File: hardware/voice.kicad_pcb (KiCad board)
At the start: 2 copper layers, 111.8 x 50.8 mm, 56 parts, among them K1 PWR, P1 DATA, P2 OUT, U1 4051, U2 MCP4922-E/P, U3 MCP4922-E/P, U4 TL074, U5 SSM2044, U6 SSM2044

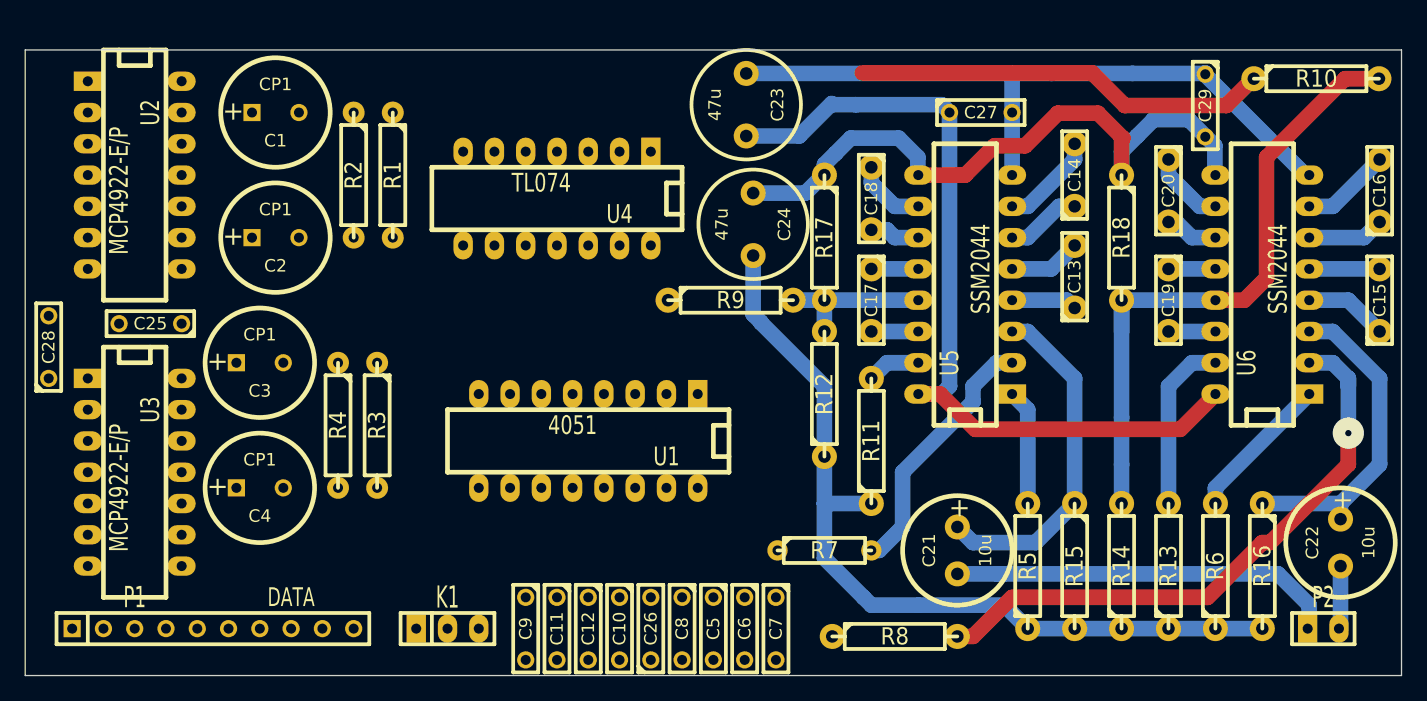
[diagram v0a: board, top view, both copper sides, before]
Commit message: hardware project cleanup
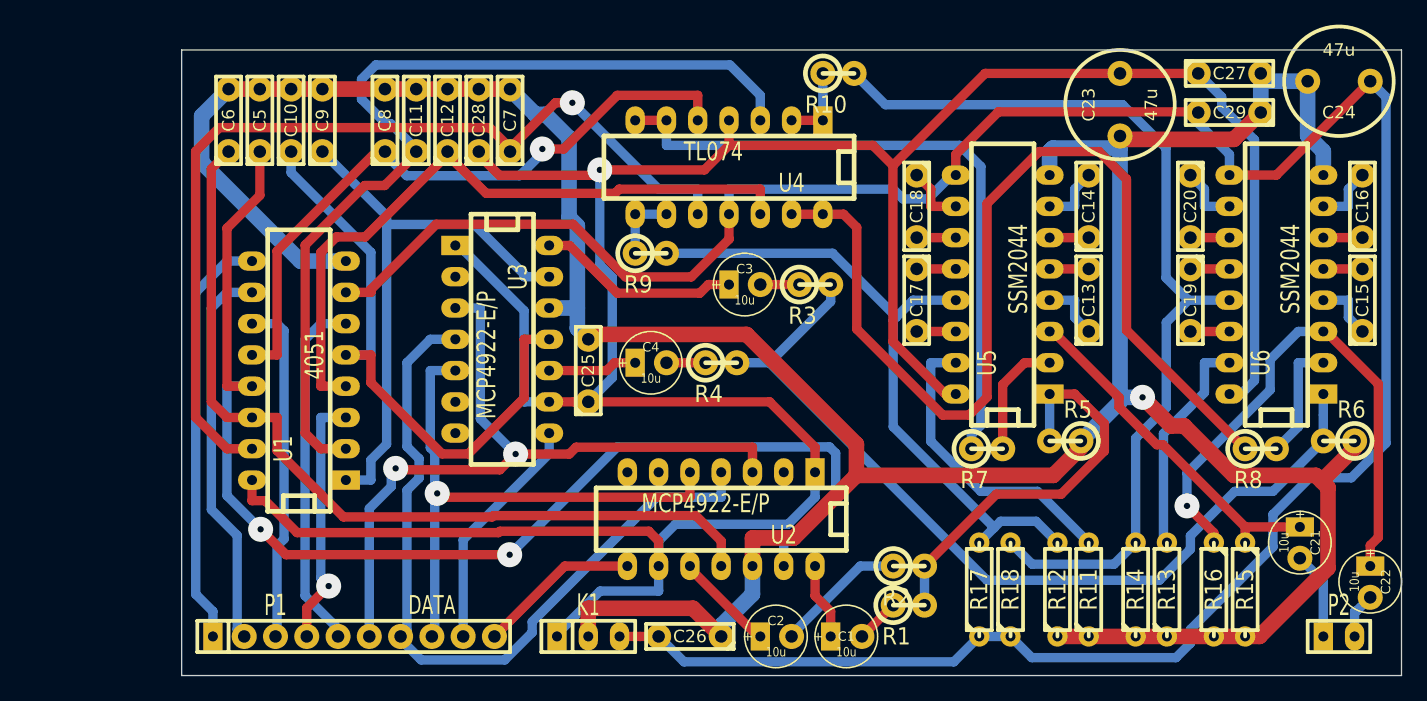
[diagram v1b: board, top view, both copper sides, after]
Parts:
- C1, C2, C3, C4: value CP1 -> 10u; footprint C1.5V8V -> C1V5
- C21, C22: footprint C1.5V8V -> C1V5
- R1, R2, R3, R4, R5, R6, R8: footprint R4-LARGE_PADS -> R1
- R10, R9: value 68k -> 6k8; footprint R4-LARGE_PADS -> R1
- R11, R12, R13, R14: footprint R4-LARGE_PADS -> R3-LARGE_PADS
- R15, R16: value 2k2 -> 3k3; footprint R4-LARGE_PADS -> R3-LARGE_PADS
- R17, R18: value 18k -> 47k; footprint R4-LARGE_PADS -> R3-LARGE_PADS
- R7: footprint R3-LARGE_PADS -> R1
- moved C1 62.9 mm to (97.2, 69.2)
- moved C6 58.8 mm to (47.0, 27.3), turned to 90 degrees
- moved C5 55.3 mm to (49.5, 27.3), turned to 90 degrees
- moved U2 55.2 mm to (87.0, 59.7), turned to 180 degrees
- moved R2 55.1 mm to (102.2, 63.5), turned to 0 degrees
- moved R1 54.6 mm to (102.2, 66.7), turned to 0 degrees
- moved C2 52.0 mm to (91.4, 69.2)
- moved C10 49.1 mm to (52.1, 27.3), turned to 90 degrees
- moved C24 49.0 mm to (137.2, 24.1), turned to 0 degrees
- moved C8 47.8 mm to (59.7, 27.3), turned to 90 degrees
- moved C7 46.6 mm to (69.8, 27.3), turned to 90 degrees
- moved C9 44.5 mm to (54.6, 27.3), turned to 90 degrees
- moved C11 42.8 mm to (62.2, 27.3), turned to 90 degrees
- moved C12 42.8 mm to (64.8, 27.3), turned to 90 degrees
- moved C3 39.9 mm to (88.9, 40.6)
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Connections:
- P1 pad 1: //LDAC_A -> N-0000041
- P1 pad 10: N-0000035 -> //LDAC_A
- P1 pad 2: //LDAC_B -> N-0000043
- P1 pad 3: /SDI -> N-0000050
- P1 pad 4: /SCK -> N-0000034
- P1 pad 5: //CS -> N-0000042
- P1 pad 6: N-0000043 -> //CS
- P1 pad 7: N-0000036 -> /SCK
- P1 pad 8: N-0000050 -> /SDI
- P1 pad 9: N-0000032 -> //LDAC_B
- U1 pad 10: N-0000036 -> N-0000043
- U1 pad 3: N-0000032 -> N-0000034
- U1 pad 6: N-0000035 -> N-0000042
- U1 pad 9: N-0000043 -> N-0000041
- U4 pad 1: N-0000015 -> N-0000045
- U4 pad 12: N-0000060 -> N-0000061
- U4 pad 13: N-0000045 -> N-0000015
- U4 pad 14: N-0000045 -> N-0000015
- U4 pad 2: N-0000015 -> N-0000045
- U4 pad 3: N-0000061 -> N-0000060
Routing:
- net +5V: track 69.5 -> 247.4 mm, vias 0 -> 1
- net -5V: track 54.5 -> 207.7 mm
- net GND: track 126.2 -> 268.5 mm, vias 0 -> 1
- net N-0000063: track 0.00 -> 99.8 mm, vias 0 -> 2
- net N-0000015: track 0.00 -> 83.7 mm
- net N-0000065: track 0.00 -> 76.2 mm, vias 0 -> 1
- net N-0000060: track 0.00 -> 75.2 mm
- net N-0000064: track 0.00 -> 70.7 mm
- net /SCK: track 0.00 -> 63.0 mm
- net //CS: track 0.00 -> 61.4 mm, vias 0 -> 2
- net N-0000046: track 12.0 -> 72.5 mm
- net N-0000061: track 0.00 -> 55.6 mm
- net N-0000048: track 0.00 -> 54.1 mm
- net N-0000062: track 0.00 -> 53.8 mm, vias 0 -> 1
- net N-0000056: track 0.00 -> 49.0 mm
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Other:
- board size 111.8 x 50.8 mm -> 99.1 x 50.8 mm
- net class Default: clearance 0.762 -> 0.508; via_dia 2.54 -> 2.032
- net class pwr added: clearance 0.508, trace_width 1.27, via_dia 2.032, via_drill 0.508
- rule trace_clearance: 0.762 -> 0.508
